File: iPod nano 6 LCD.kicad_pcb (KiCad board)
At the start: 2 copper layers, 119.4 x 46.2 mm, 108 parts, among them J1 Molex_503548-1220, J2 USB_C_Receptacle_USB2.0, SW1 SW_Push, SW2 SW_Push, U1 AP5724, U2 ICE40HX1K-TQ144, U3 TLV62569DBV, U4 TLV62569DBV, U5 XTSD04GLGEAG, U6 TLV62569DBV, U7 AT25xxx, U8 USBLC6-2P6, U9 FT232H, Y1 12MHz

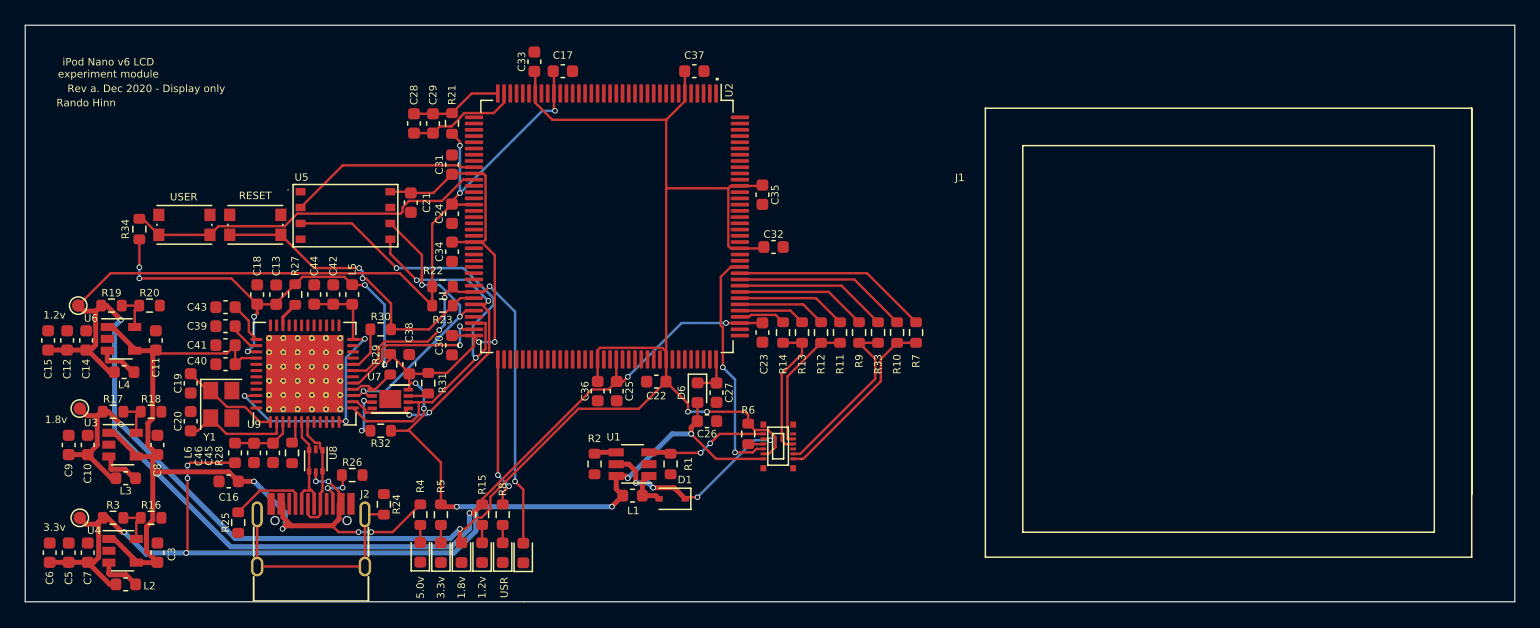
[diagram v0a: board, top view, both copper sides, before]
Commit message: Nearly done with routing.
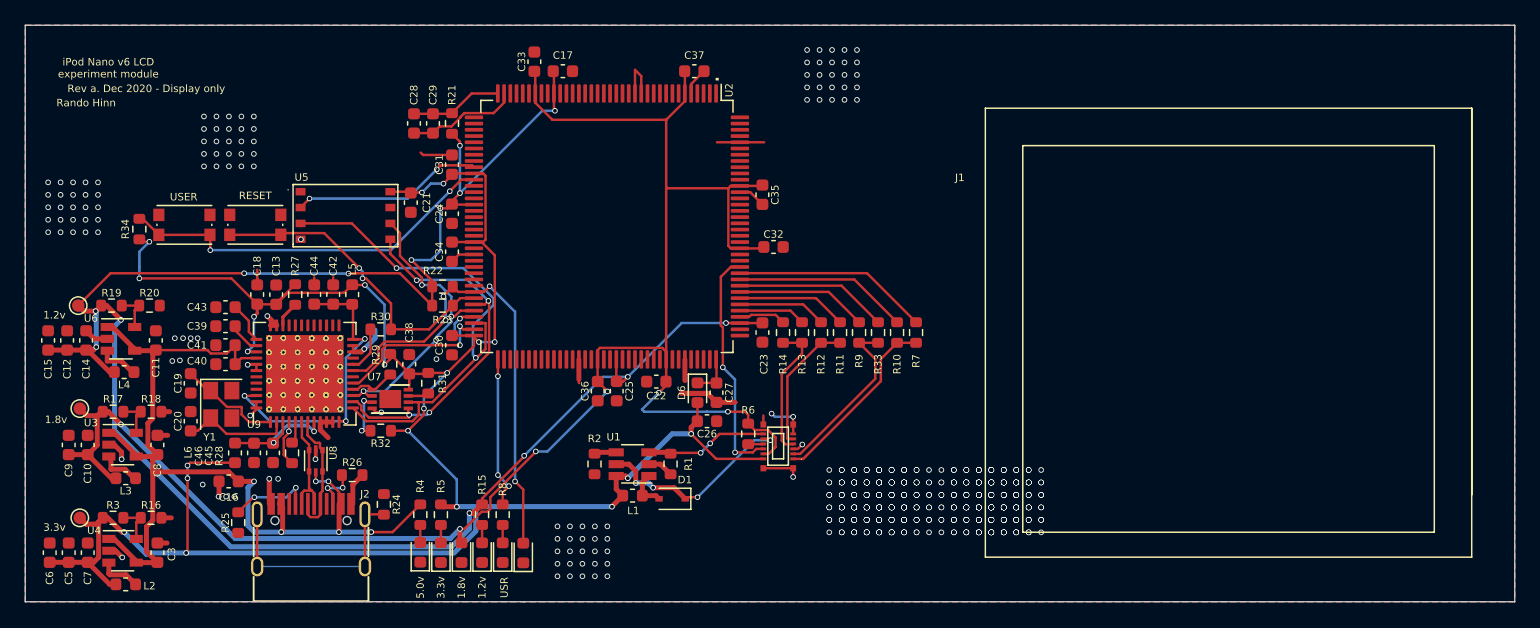
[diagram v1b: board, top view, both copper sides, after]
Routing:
- net GND: track 0.00 -> 75.9 mm, vias 0 -> 628
- net Net-(C45-Pad2): track 5.08 -> 12.9 mm, vias 0 -> 2
- net +1V2: track 149.7 -> 154.1 mm, vias 7 -> 14
- net +3V3: track 180.3 -> 184.5 mm, vias 18 -> 21
- net +5V: track 76.5 -> 78.9 mm
- net Net-(R34-Pad2): track 29.4 -> 30.9 mm, vias 0 -> 2
- net MOSI: track 30.7 -> 31.3 mm
- net Net-(J2-PadA5): track 6.26 -> 6.75 mm, vias 0 -> 2
- net MISO: track 25.1 -> 25.4 mm, vias 3 -> 4
- net +1V8: track 143.3 -> 143.1 mm, vias 4 -> 6
- net SD_CS: vias 0 -> 2
- net /USR_LED: vias 2 -> 3
- added copper zone on B.Cu, net GND
- added copper zone on F.Cu, net GND
